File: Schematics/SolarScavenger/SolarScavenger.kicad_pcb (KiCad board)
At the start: 2 copper layers, 38 parts, among them J1 SolarConnector, J10 CH1_OUT, J11 CH2_OUT, J12 CH3_OUT, J13 CH4_OUT, J2 PROGRAMMING, J3 BatteryPack, J4 ESC_PWM_CONTROL, J5 ESC_connector, J6 CH1_IN, J7 CH2_IN, J8 CH3_IN, J9 CH4_IN, Q1 IRLML2502, Q2 IRLML2502, U1 4N25, U2 AP1117-33, U3 ESP32-WROOM-E, U4 INA219AxD

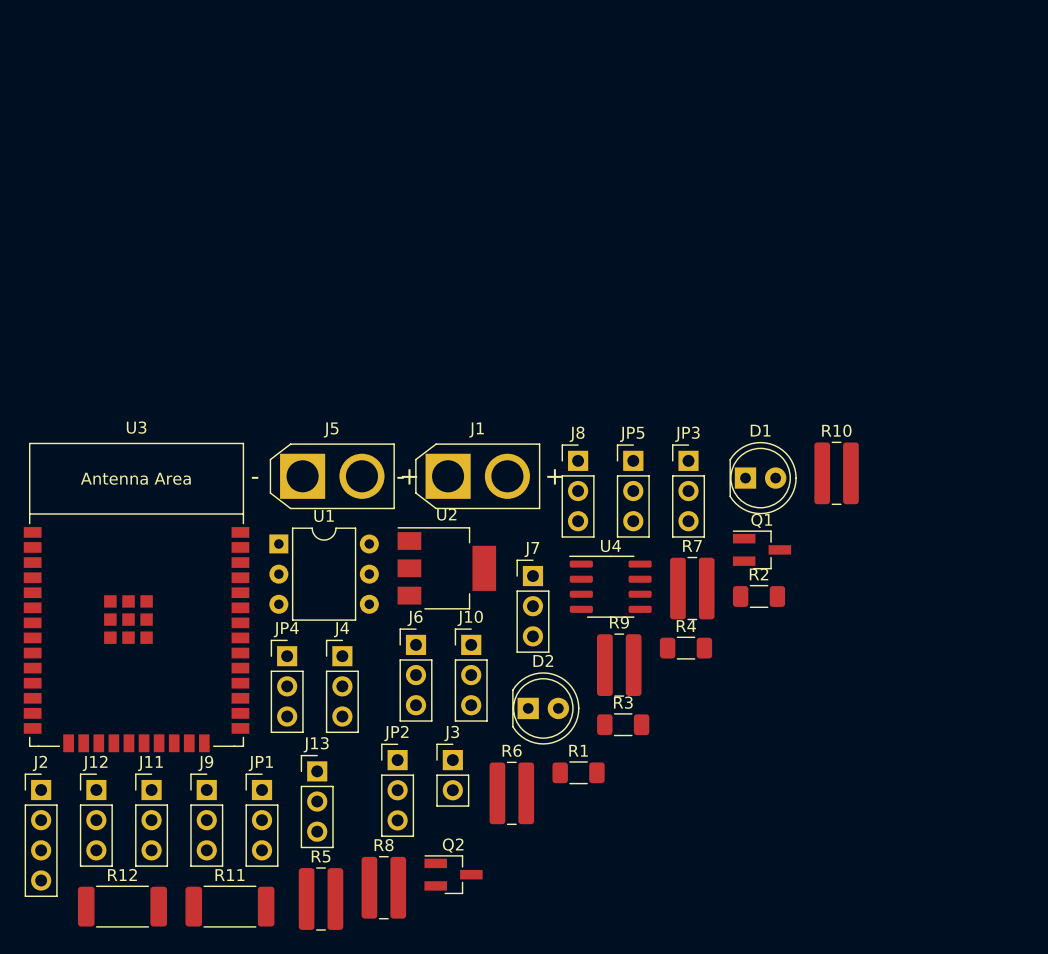
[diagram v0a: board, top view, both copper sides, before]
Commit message: PCB final candidate
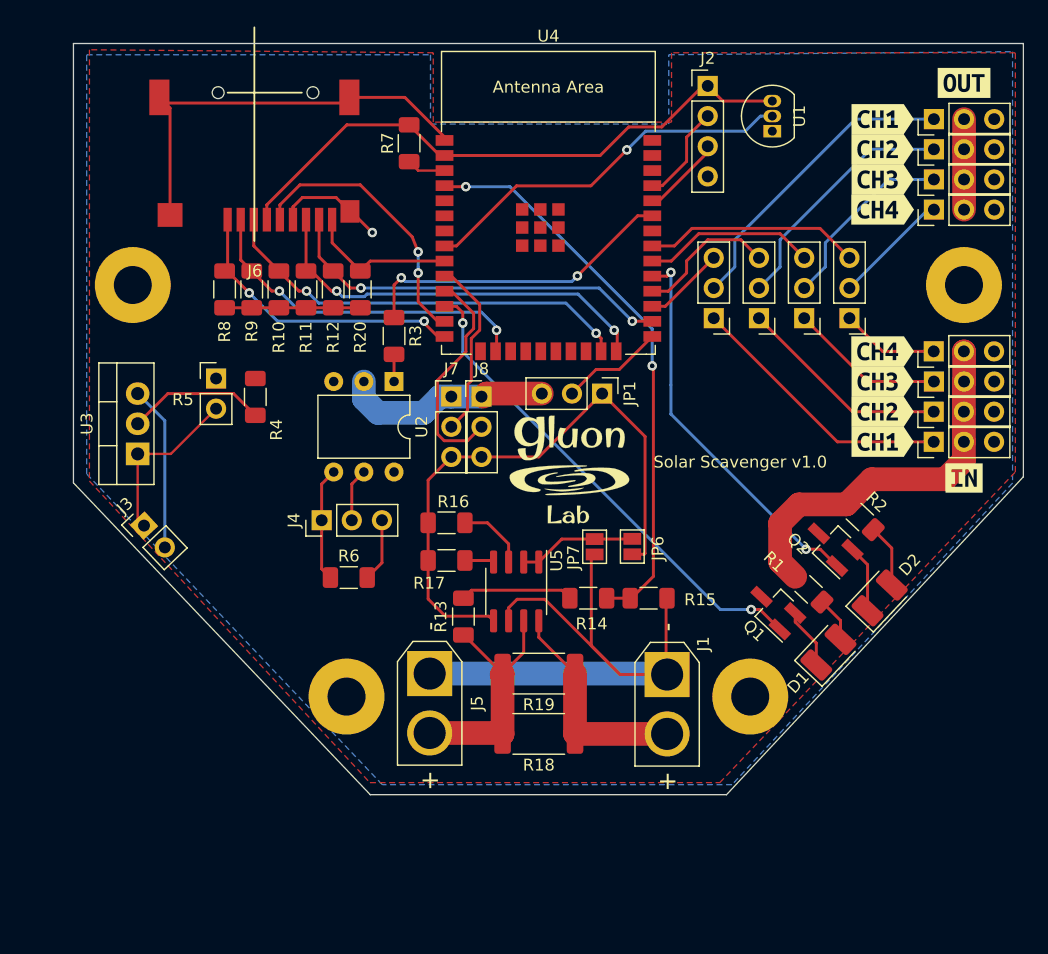
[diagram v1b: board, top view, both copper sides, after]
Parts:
- removed J9: CH4_IN, Connector_PinHeader_2.54mm:PinHeader_1x03_P2.54mm_Vertical
- added G***: LOGO, GluonLib:LogoGluon_12mm, F.Cu at (141.7, 68.6)
- added J14: CH1_OUT, Connector_PinHeader_2.54mm:PinHeader_1x03_P2.54mm_Vertical, F.Cu at (172.5, 39.4)
- added J15: CH2_OUT, Connector_PinHeader_2.54mm:PinHeader_1x03_P2.54mm_Vertical, F.Cu at (172.5, 41.9)
- added J16: CH3_OUT, Connector_PinHeader_2.54mm:PinHeader_1x03_P2.54mm_Vertical, F.Cu at (172.5, 44.5)
- added J17: CH4_OUT, Connector_PinHeader_2.54mm:PinHeader_1x03_P2.54mm_Vertical, F.Cu at (172.5, 47.0)
- added JP6: INA_A0, Jumper:SolderJumper-2_P1.3mm_Open_Pad1.0x1.5mm, F.Cu at (147.1, 75.4)
- added JP7: INA_A1, Jumper:SolderJumper-2_P1.3mm_Open_Pad1.0x1.5mm, F.Cu at (143.9, 75.4)
- added R13: 1k, Resistor_SMD:R_1206_3216Metric_Pad1.30x1.75mm_HandSolder, F.Cu at (132.8, 81.3)
- added R14: 1k, Resistor_SMD:R_1206_3216Metric_Pad1.30x1.75mm_HandSolder, F.Cu at (143.4, 79.7)
- added R15: 330, Resistor_SMD:R_1206_3216Metric_Pad1.30x1.75mm_HandSolder, F.Cu at (148.4, 79.7)
- added R16: 1k, Resistor_SMD:R_1206_3216Metric_Pad1.30x1.75mm_HandSolder, F.Cu at (131.4, 73.4)
- added R17: 1k, Resistor_SMD:R_1206_3216Metric_Pad1.30x1.75mm_HandSolder, F.Cu at (131.4, 76.5)
- added R18: R100/2W, Resistor_SMD:R_2512_6332Metric_Pad1.40x3.35mm_HandSolder, F.Cu at (139.2, 91.1)
- added R19: R100/2W, Resistor_SMD:R_2512_6332Metric_Pad1.40x3.35mm_HandSolder, F.Cu at (139.2, 86.1)
- added R20: 47k, Resistor_SMD:R_1206_3216Metric_Pad1.30x1.75mm_HandSolder, F.Cu at (124.2, 53.7)
- added REF**: MountingHole_3.2mm_M3_Pad, MountingHole:MountingHole_3.2mm_M3_Pad, F.Cu at (105.0, 53.3)
- added REF**: MountingHole_3.2mm_M3_Pad, MountingHole:MountingHole_3.2mm_M3_Pad, F.Cu at (175.0, 53.3)
- added REF**: MountingHole_3.2mm_M3_Pad, MountingHole:MountingHole_3.2mm_M3_Pad, F.Cu at (123.0, 88.0)
- added REF**: MountingHole_3.2mm_M3_Pad, MountingHole:MountingHole_3.2mm_M3_Pad, F.Cu at (157.0, 88.0)
- added U5: INA219AxD, Package_SO:SOIC-8_3.9x4.9mm_P1.27mm, F.Cu at (137.3, 79.1)
- added kibuzzard-63EE93D3: G***, kibuzzard-63EE93D3, F.Cu at (168.1, 66.5)
- added kibuzzard-63EE93FE: G***, kibuzzard-63EE93FE, F.Cu at (168.1, 64.0)
- added kibuzzard-63EE93FE: G***, kibuzzard-63EE93FE, F.Cu at (168.1, 41.9)
- added kibuzzard-63EE940D: G***, kibuzzard-63EE940D, F.Cu at (168.1, 39.4)
- added kibuzzard-63EE941D: G***, kibuzzard-63EE941D, F.Cu at (168.1, 61.5)
- added kibuzzard-63EE9442: G***, kibuzzard-63EE9442, F.Cu at (168.1, 44.5)
- added kibuzzard-63EE9448: G***, kibuzzard-63EE9448, F.Cu at (168.1, 58.9)
- added kibuzzard-63EE9448: G***, kibuzzard-63EE9448, F.Cu at (168.1, 47.0)
- added kibuzzard-63F118E7: G***, kibuzzard-63F118E7, F.Cu at (175.0, 36.3)
- added kibuzzard-63F118F7: G***, kibuzzard-63F118F7, F.Cu at (175.0, 69.6)
- D1, D2: footprint LED_THT:LED_D5.0mm -> LED_SMD:LED_1210_3225Metric_Pad1.42x2.65mm_HandSolder
- J10: value CH1_OUT -> CH1_IN
- J11: value CH2_OUT -> CH2_IN
- J12: value CH3_OUT -> CH3_IN
- J13: value CH4_OUT -> CH4_IN
- J6: value CH1_IN -> Micro_SD_Card; footprint Connector_PinHeader_2.54mm:PinHeader_1x03_P2.54mm_Vertical -> microSD:microSD-Receptacle-SelfEject
- J7: value CH2_IN -> RUDDER_POT
- J8: value CH3_IN -> THROTTLE_POt
- R1: value 220 -> 300
- R10, R9: value 1k -> 47k; footprint Resistor_SMD:R_1020_2550Metric_Pad1.33x5.20mm_HandSolder -> Resistor_SMD:R_1206_3216Metric_Pad1.30x1.75mm_HandSolder
- R11, R12: value R100/2W -> 47k; footprint Resistor_SMD:R_2512_6332Metric_Pad1.40x3.35mm_HandSolder -> Resistor_SMD:R_1206_3216Metric_Pad1.30x1.75mm_HandSolder
- R3: value 300 -> 220
- R4: value 1k -> 4k7
- R5: value 10k -> R_Photo; footprint Resistor_SMD:R_1020_2550Metric_Pad1.33x5.20mm_HandSolder -> Connector_PinHeader_2.54mm:PinHeader_1x02_P2.54mm_Vertical
- R6: footprint Resistor_SMD:R_1020_2550Metric_Pad1.33x5.20mm_HandSolder -> Resistor_SMD:R_1206_3216Metric_Pad1.30x1.75mm_HandSolder
- R7: value 1k -> 10k; footprint Resistor_SMD:R_1020_2550Metric_Pad1.33x5.20mm_HandSolder -> Resistor_SMD:R_1206_3216Metric_Pad1.30x1.75mm_HandSolder
- R8: value 330 -> 47k; footprint Resistor_SMD:R_1020_2550Metric_Pad1.33x5.20mm_HandSolder -> Resistor_SMD:R_1206_3216Metric_Pad1.30x1.75mm_HandSolder
- U1: value 4N25 -> DS18B20; footprint Package_DIP:DIP-6_W7.62mm -> Package_TO_SOT_THT:TO-92_Inline
- U2: value AP1117-33 -> 4N25; footprint Package_TO_SOT_SMD:SOT-223-3_TabPin2 -> Package_DIP:DIP-6_W7.62mm
- U3: value ESP32-WROOM-E -> AP1117-33; footprint Espressif:ESP32-WROOM-32E -> Package_TO_SOT_THT:TO-220-3_Vertical
- U4: value INA219AxD -> ESP32-WROOM-E; footprint Package_SO:SOIC-8_3.9x4.9mm_P1.27mm -> Espressif:ESP32-WROOM-32E
- moved J2 81.7 mm to (153.4, 36.6)
- moved J12 78.5 mm to (172.5, 61.5), turned to 90 degrees
- moved J11 73.2 mm to (172.5, 64.0), turned to 90 degrees
- moved J13 62.8 mm to (172.5, 58.9), turned to 90 degrees
- moved R12 54.9 mm to (121.9, 53.7), turned to -90 degrees
- moved U1 54.2 mm to (158.9, 40.4), turned to 90 degrees
- moved R11 52.4 mm to (119.6, 53.7), turned to -90 degrees
- moved R8 52.1 mm to (112.7, 53.7), turned to -90 degrees
- moved JP4 52.0 mm to (161.5, 56.1), turned to 180 degrees
- moved R10 49.5 mm to (117.3, 53.7), turned to -90 degrees
- moved JP2 45.8 mm to (153.9, 56.1), turned to 180 degrees
- moved R5 44.7 mm to (112.0, 61.2)
- moved R7 44.4 mm to (128.3, 41.4), turned to 90 degrees
- moved R9 44.3 mm to (115.0, 53.7), turned to -90 degrees
- moved JP1 44.0 mm to (144.5, 62.5), turned to -90 degrees
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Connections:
- D1 pad 2: Net-(D1-Pad2) -> Net-(D1-A)
- D2 pad 2: Net-(D2-Pad2) -> Net-(D2-A)
- J1 pad 1: SUPPLY_IN_P -> MOTOR_SUPPLY_N
- J1 pad 2: MOTOR_SUPPLY_N -> SUPPLY_IN_P
- J10 pad 1: Net-(J10-Pad1) -> Net-(J10-Pin_1)
- J11 pad 1: Net-(J11-Pad1) -> Net-(J11-Pin_1)
- J12 pad 1: Net-(J12-Pad1) -> Net-(J12-Pin_1)
- J13 pad 1: Net-(J13-Pad1) -> Net-(J13-Pin_1)
- J3 pad 2: Net-(J3-Pad2) -> Net-(J3-Pin_2)
- J5 pad 1: MOTOR_SUPPLY_P -> MOTOR_SUPPLY_N
- J5 pad 2: MOTOR_SUPPLY_N -> MOTOR_SUPPLY_P
- J6 pad 1: Net-(J6-Pad1) -> /SD_DATA2
- J6 pad 2: ESC_5V -> /SD_DATA3
- J6 pad 3: MOTOR_SUPPLY_N -> /SD_CMD
- J7 pad 1: Net-(J7-Pad1) -> MOTOR_SUPPLY_N
- J7 pad 2: ESC_5V -> RUDDER_ADC
- J7 pad 3: MOTOR_SUPPLY_N -> +3V3
- J8 pad 1: Net-(J8-Pad1) -> MOTOR_SUPPLY_N
- J8 pad 2: ESC_5V -> THROTTLE_ADC
- J8 pad 3: MOTOR_SUPPLY_N -> +3V3
- JP2 pad 1: Net-(J6-Pad1) -> Net-(J10-Pin_1)
- JP2 pad 2: Net-(J10-Pad1) -> Net-(J14-Pin_1)
- JP3 pad 1: Net-(J7-Pad1) -> Net-(J11-Pin_1)
- JP3 pad 2: Net-(J11-Pad1) -> Net-(J15-Pin_1)
- JP4 pad 1: Net-(J8-Pad1) -> Net-(J12-Pin_1)
- JP4 pad 2: Net-(J12-Pad1) -> Net-(J16-Pin_1)
- JP5 pad 1: Net-(J9-Pad1) -> Net-(J13-Pin_1)
- JP5 pad 2: Net-(J13-Pad1) -> Net-(J17-Pin_1)
- R1 pad 1: PWM_TO_ESC -> ESC_5V
- R1 pad 2: Net-(R1-Pad2) -> Net-(D1-A)
- R10 pad 1: INA_SCL -> /SD_CMD
- R11 pad 1: SUPPLY_IN_P -> /SD_DATA0
- R11 pad 2: MOTOR_SUPPLY_P -> +3V3
- R12 pad 1: SUPPLY_IN_P -> /SD_DATA1
- R12 pad 2: MOTOR_SUPPLY_P -> +3V3
- R2 pad 2: Net-(D1-Pad2) -> Net-(D2-A)
- R3 pad 1: ESC_5V -> PWM_TO_ESC
- R3 pad 2: Net-(D2-Pad2) -> Net-(R3-Pad2)
- R4 pad 1: ESC_PWM -> +3V3
- R4 pad 2: ESC_GND -> LIGHT_SENSOR
- R5 pad 1: MOTOR_SUPPLY_N -> LIGHT_SENSOR
- R5 pad 2: +3V3 -> MOTOR_SUPPLY_N
- R6 pad 1: Net-(R6-Pad1) -> ESC_PWM
- R6 pad 2: MOTOR_SUPPLY_P -> ESC_GND
- R7 pad 1: MOTOR_VOLTAGE -> MOTOR_SUPPLY_N
- R7 pad 2: Net-(R6-Pad1) -> +3V3
- R8 pad 1: MOTOR_SUPPLY_N -> /SD_DATA2
- R8 pad 2: MOTOR_VOLTAGE -> +3V3
- R9 pad 1: +3V3 -> /SD_DATA3
- R9 pad 2: INA_SDA -> +3V3
- U1 pad 1: Net-(R1-Pad2) -> MOTOR_SUPPLY_N
- U1 pad 2: MOTOR_SUPPLY_N -> TEMP_SENSOR
- U1 pad 3: unconnected-(U1-Pad3) -> +3V3
- U2 pad 1: MOTOR_SUPPLY_N -> Net-(R3-Pad2)
- U2 pad 2: +3V3 -> MOTOR_SUPPLY_N
- U2 pad 3: Net-(J3-Pad2) -> unconnected-(U2-NC-Pad3)
- U3 pad 3: MOTOR_SUPPLY_N -> Net-(J3-Pin_2)
- U4 pad 1: +3V3 -> MOTOR_SUPPLY_N
- U4 pad 3: INA_SDA -> MOTOR_SUPPLY_N
- U4 pad 4: INA_SCL -> MOTOR_VOLTAGE
- U4 pad 5: +3V3 -> LIGHT_SENSOR
- U4 pad 6: MOTOR_SUPPLY_N -> unconnected-(U4-GPIO34/ADC1_CH6-Pad6)
- U4 pad 7: MOTOR_SUPPLY_P -> unconnected-(U4-GPIO35/ADC1_CH7-Pad7)
- U4 pad 8: SUPPLY_IN_P -> TEMP_SENSOR
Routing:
- net MOTOR_SUPPLY_N: track 0.00 -> 135.6 mm, vias 0 -> 1
- net +3V3: track 0.00 -> 123.8 mm
- net MOTOR_VOLTAGE: track 0.00 -> 48.1 mm, vias 0 -> 2
- net ESC_5V: track 0.00 -> 44.0 mm
- net LED_2: track 0.00 -> 41.4 mm, vias 0 -> 2
- net /SD_CMD: track 0.00 -> 35.8 mm, vias 0 -> 2
- net /SD_DATA0: track 0.00 -> 34.4 mm, vias 0 -> 2
- net /SD_DATA1: track 0.00 -> 33.4 mm, vias 0 -> 2
- net LED_1: track 0.00 -> 32.9 mm, vias 0 -> 2
- net TEMP_SENSOR: track 0.00 -> 32.1 mm, vias 0 -> 1
- net /SD_DATA3: track 0.00 -> 29.3 mm, vias 0 -> 2
- net PWM_TO_ESC: track 0.00 -> 27.2 mm, vias 0 -> 2
- net Net-(J14-Pin_1): track 0.00 -> 25.8 mm
- net /SD_DATA2: track 0.00 -> 25.3 mm, vias 0 -> 2
- net /SD_CLK: track 0.00 -> 23.4 mm, vias 0 -> 2
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- added copper zone on B.Cu, net MOTOR_SUPPLY_N
- added copper zone on F.Cu, net MOTOR_SUPPLY_N
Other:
- board outline added: 80 x 63.3 mm
- board text added: "Solar Scavenger v1.0"
